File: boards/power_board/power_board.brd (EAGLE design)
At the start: 75 x 50 mm, 24 parts, among them J5 USB_A_SMT_FEMALE, J6 USB_A_SMT_FEMALE, Q2 IRFR5305, U1 YZXSTUDIO_SOLARCHARGERDEFAULT, U2 PTH08080WPTH08080W, U3 MAX2812MAX2812_SOIC8

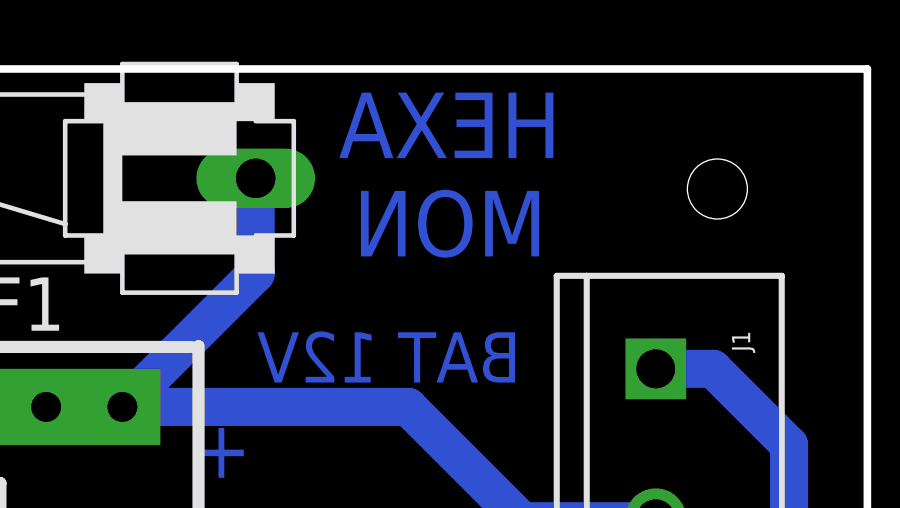
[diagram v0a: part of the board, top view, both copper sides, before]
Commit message: Minor modifications, images of board & schema included
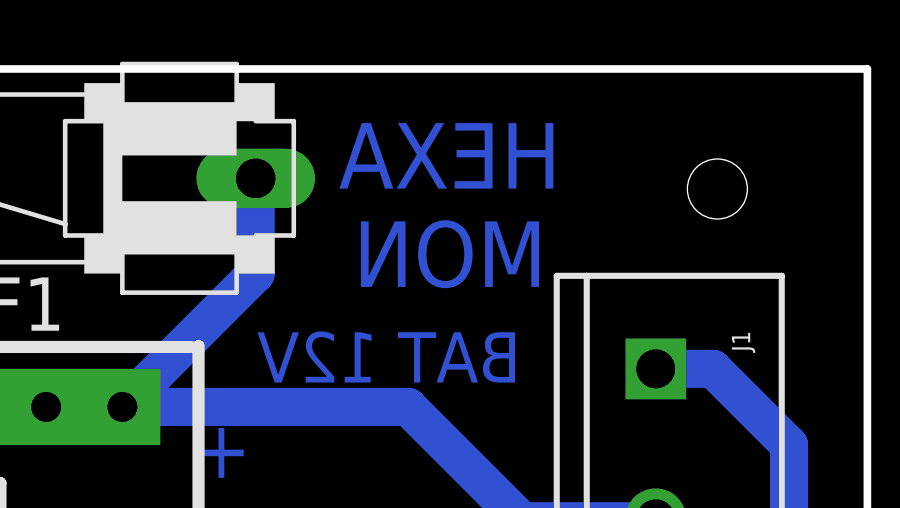
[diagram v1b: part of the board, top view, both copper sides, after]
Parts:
- R4: value 3M9 -> 3M3
- R6: value 370k -> 470k
- R7: value 820k -> 120k
- R8: value 100 -> 0
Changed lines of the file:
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@@
 <hole x="70" y="46" drill="2"/>
 <hole x="4" y="4" drill="2"/>
-<text x="61.087" y="46.482" size="2.1844" layer="16" font="vector" ratio="15" rot="MR180" align="center">HEXA
+<text x="61.087" y="45.466" size="2.1844" layer="16" font="vector" ratio="15" rot="MR180" align="center">HEXA
 MON</text>
 <text x="39.243" y="38.354" size="1.9304" layer="16" font="vector" ratio="15" rot="MR180" align="center">+</text>
@@
 <element name="R2" library="rcl" package="R1206" value="1M" x="22.606" y="20.701" rot="MR180"/>
 <element name="R3" library="rcl" package="R1206" value="1M" x="41.656" y="27.813" rot="MR0"/>
-<element name="R4" library="rcl" package="R1206" value="3M9" x="31.115" y="38.735" rot="MR270"/>
-<element name="R6" library="rcl" package="R1206" value="370k" x="33.655" y="29.21" rot="MR180"/>
+<element name="R4" library="rcl" package="R1206" value="3M3" x="31.115" y="38.735" rot="MR270"/>
+<element name="R6" library="rcl" package="R1206" value="470k" x="33.655" y="29.21" rot="MR180"/>
 <element name="F1" library="special" package="FUSE" value="3A" x="43.18" y="46.355" rot="R180"/>
 <element name="J5" library="SparkFun-Connectors" package="USB-A-S-SILK-FEMALE" value="USB_A_SMT_FEMALE" x="47.625" y="6.985" rot="MR90">
@@
 </element>
 <element name="U3" library="custom_adluc" package="SOIC127P600X175-8N" value="MAX2812MAX2812_SOIC8" x="24.765" y="31.75" rot="MR0"/>
-<element name="R8" library="rcl" package="R1206" value="100" x="14.859" y="38.735" rot="MR180"/>
-<element name="R7" library="rcl" package="R1206" value="820k" x="27.94" y="38.735" rot="MR90"/>
+<element name="R8" library="rcl" package="R1206" value="0" x="14.859" y="38.735" rot="MR180"/>
+<element name="R7" library="rcl" package="R1206" value="120k" x="27.94" y="38.735" rot="MR90"/>
 <element name="R5" library="rcl" package="RTRIM64Y" value="1M" x="20.955" y="44.45" rot="R90"/>
 <element name="C1" library="rcl" package="E3,5-8" value="100u" x="38.1" y="34.925" rot="R270"/>
